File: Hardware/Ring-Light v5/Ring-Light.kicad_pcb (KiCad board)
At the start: 4 copper layers, 115 x 146.1 mm, 319 parts, among them J1 694106301002, J2 1017457000B11LF, J3 U.FL-R-SMT-1_80, J4 2002112100010C4LF, J5 640445-2, J6 Conn_01x01, J7 Conn_01x01, J8 Conn_01x01, J9 Conn_01x01, Q1 SQJ415EP-T1_GE3, U1 NCR321PASX, U10 NCR321PASX, U11 NCR321PASX, U12 NCR321PASX, U13 NCR321PASX, U14 NCR321PASX, U15 NCR321PASX, U16 NCR321PASX, U17 NCR321PASX, U18 NCR321PASX, U19 NCR321PASX, U2 NCR321PASX, U20 NCR321PASX, U21 NCR321PASX, U22 NCR321PASX, U23 NCR321PASX, U24 NCR321PASX, U25 NCR321PASX, U26 NCR321PASX, U27 NCR321PASX, U28 NCR321PASX, U29 NCR321PASX, U3 NCR321PASX, U30 NCR321PASX, U31 NCR321PASX, U32 NCR321PASX, U33 PCA9685BS,118, U34 PCA9685BS,118, U36 TPS62177DQC, U37 CP2102N-A02-GQFN20R, U38 W25X40CLUXIG_TR, U39 CC2640R2FRGZR, U4 NCR321PASX, U5 NCR321PASX, U6 NCR321PASX, U7 NCR321PASX, U8 NCR321PASX, U9 NCR321PASX, Y1 32.768kHz, Y2 24MHz

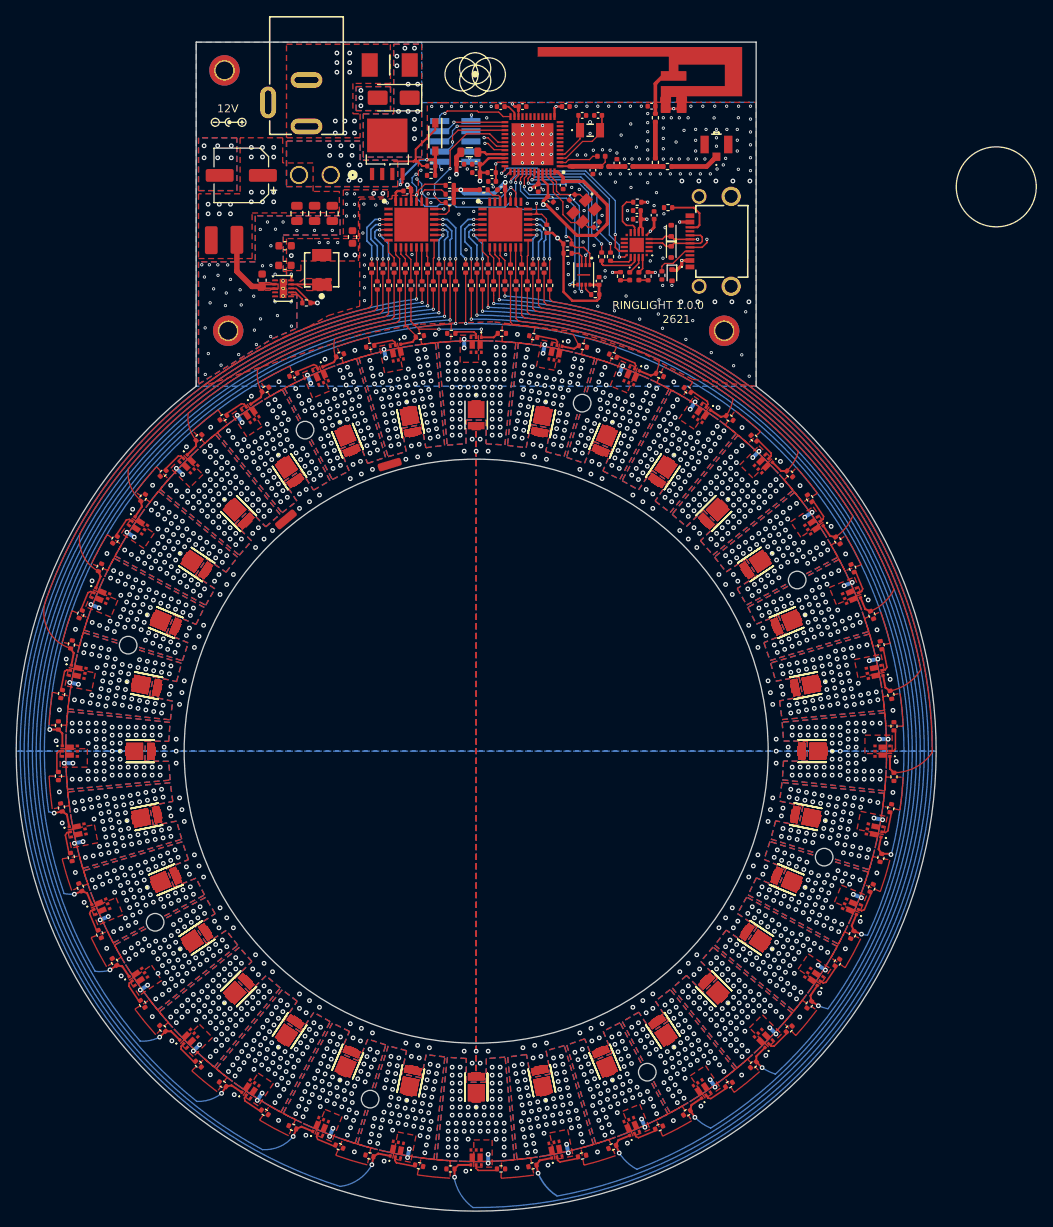
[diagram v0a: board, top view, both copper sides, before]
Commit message: m
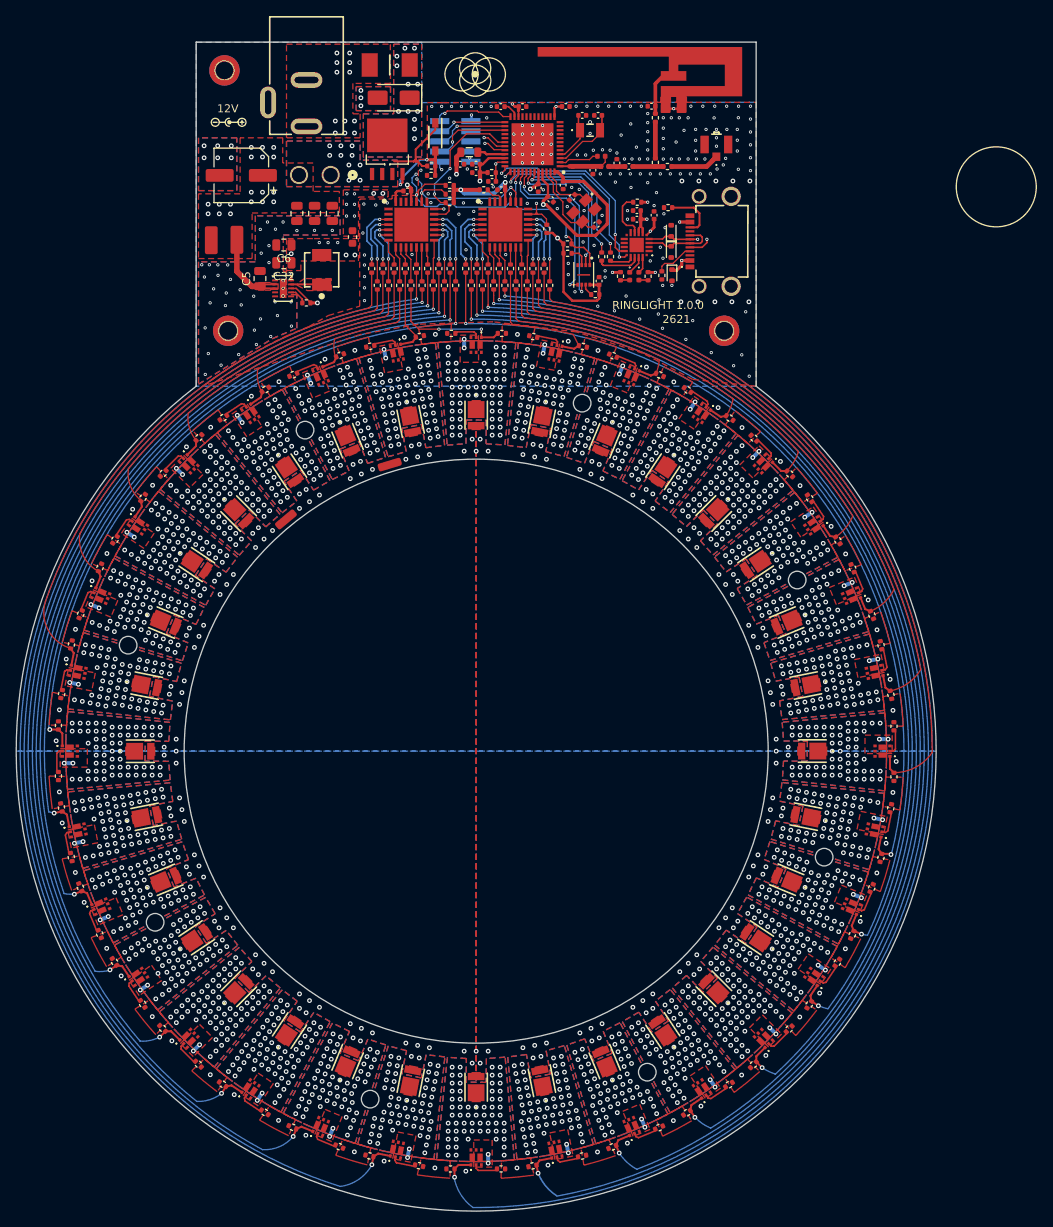
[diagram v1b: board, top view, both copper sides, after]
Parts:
- removed the D10 at (52.9, 126.9) (x2)
- removed the D11 at (55.3, 134.7)
- removed the D12 at (59.2, 142.0)
- removed the D13 at (64.4, 148.4)
- removed the D14 at (70.8, 153.6)
- removed the D15 at (78.1, 157.5)
- removed the D16 at (85.9, 159.9)
- removed the D17 at (94.1, 160.7)
- removed the D18 at (102.3, 159.9)
- removed the D19 at (110.2, 157.5)
- removed the D2 at (85.9, 77.5) (x2)
- removed the D20 at (117.5, 153.6)
- removed the D21 at (123.8, 148.4)
- removed the D22 at (129.0, 142.0) (x2)
- removed the D23 at (132.9, 134.7)
- removed the D24 at (135.3, 126.9) (x2)
- removed the D25 at (136.1, 118.7) (x2)
- removed the D26 at (135.3, 110.5) (x2)
- removed the D27 at (132.9, 102.6) (x2)
- removed the D28 at (129.0, 95.3)
- removed the D29 at (123.8, 89.0)
- removed the D3 at (78.0, 79.9)
- removed the D30 at (117.4, 83.7) (x2)
- removed the D31 at (110.2, 79.9)
- removed the D32 at (102.3, 77.5)
- removed the D4 at (70.8, 83.7)
- removed the D4 at (70.8, 83.8)
- removed D41, D45, D47, D49, D50, D51, D52, D53, D54, D55, D56, D57, D58, D59, D61, D66, D67, D69, D70: LED, Library:GWJTLRS1EMLVL5XX531
- removed the D5 at (64.4, 89.0) (x2)
- removed the D6 at (59.2, 95.3) (x2)
- removed the D7 at (55.3, 102.6)
- removed the D8 at (52.9, 110.5) (x2)
- removed the D9 at (52.1, 118.7)
- C1, C2, C7, C8: value 0.1uF -> 100nF
- C20: value 1.0uF -> 1uF
- C32, C6: footprint Capacitor_SMD:C_0603_1608Metric -> Capacitor_SMD:C_0805_2012Metric
- C5: value 0.1uF -> 2.2uF; footprint Capacitor_SMD:C_0603_1608Metric -> Capacitor_SMD:C_0805_2012Metric
- moved C32 0.35 mm to (70.1, 57.6)
- moved C5 0.34 mm to (67.1, 59.6)
- moved C6 0.18 mm to (70.1, 55.4)
- renumbered D48 to D10, D60 to D22, D62 to D24, D63 to D25, D64 to D26, D65 to D27, D68 to D30, D42 to D4, D43 to D5, D44 to D6, D46 to D8
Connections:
- D10 pad 1: /LEDs_1-16/OUT1 -> /LEDs_1-16/OUT10
- D10 pad 2: /LEDs_1-16/OUT1 -> /LEDs_1-16/OUT10
- D11 pad 1: /LEDs_1-16/OUT1 -> /LEDs_1-16/OUT11
- D11 pad 2: /LEDs_1-16/OUT1 -> /LEDs_1-16/OUT11
- D13 pad 1: /LEDs_1-16/OUT1 -> /LEDs_1-16/OUT13
- D13 pad 2: /LEDs_1-16/OUT1 -> /LEDs_1-16/OUT13
- D16 pad 1: /LEDs_1-16/OUT1 -> /LEDs_1-16/OUT16
- D16 pad 2: /LEDs_1-16/OUT1 -> /LEDs_1-16/OUT16
- D18 pad 1: /LEDs_1-16/OUT1 -> /LEDs_17-32/OUT18
- D18 pad 2: /LEDs_1-16/OUT1 -> /LEDs_17-32/OUT18
- D2 pad 1: /LEDs_1-16/OUT1 -> /LEDs_1-16/OUT2
- D2 pad 2: /LEDs_1-16/OUT1 -> /LEDs_1-16/OUT2
- D21 pad 1: /LEDs_1-16/OUT1 -> /LEDs_17-32/OUT21
- D21 pad 2: /LEDs_1-16/OUT1 -> /LEDs_17-32/OUT21
- D22 pad 1: /LEDs_1-16/OUT1 -> /LEDs_17-32/OUT22
- D22 pad 2: /LEDs_1-16/OUT1 -> /LEDs_17-32/OUT22
- D23 pad 1: /LEDs_1-16/OUT1 -> /LEDs_17-32/OUT23
- D23 pad 2: /LEDs_1-16/OUT1 -> /LEDs_17-32/OUT23
- D24 pad 1: /LEDs_1-16/OUT1 -> /LEDs_17-32/OUT24
- D24 pad 2: /LEDs_1-16/OUT1 -> /LEDs_17-32/OUT24
- D25 pad 1: /LEDs_1-16/OUT1 -> /LEDs_17-32/OUT25
- D25 pad 2: /LEDs_1-16/OUT1 -> /LEDs_17-32/OUT25
- D26 pad 1: /LEDs_1-16/OUT1 -> /LEDs_17-32/OUT26
- D26 pad 2: /LEDs_1-16/OUT1 -> /LEDs_17-32/OUT26
- D27 pad 1: /LEDs_1-16/OUT1 -> /LEDs_17-32/OUT27
- D27 pad 2: /LEDs_1-16/OUT1 -> /LEDs_17-32/OUT27
- D28 pad 1: /LEDs_1-16/OUT1 -> /LEDs_17-32/OUT28
- D28 pad 2: /LEDs_1-16/OUT1 -> /LEDs_17-32/OUT28
- D29 pad 1: /LEDs_1-16/OUT1 -> /LEDs_17-32/OUT29
- D29 pad 2: /LEDs_1-16/OUT1 -> /LEDs_17-32/OUT29
- D30 pad 1: /LEDs_1-16/OUT1 -> /LEDs_17-32/OUT30
- D30 pad 2: /LEDs_1-16/OUT1 -> /LEDs_17-32/OUT30
- D32 pad 1: /LEDs_1-16/OUT1 -> /LEDs_17-32/OUT32
- D32 pad 2: /LEDs_1-16/OUT1 -> /LEDs_17-32/OUT32
- D4 pad 1: /LEDs_1-16/OUT1 -> /LEDs_1-16/OUT4
- D4 pad 2: /LEDs_1-16/OUT1 -> /LEDs_1-16/OUT4
- D5 pad 1: /LEDs_1-16/OUT1 -> /LEDs_1-16/OUT5
- D5 pad 2: /LEDs_1-16/OUT1 -> /LEDs_1-16/OUT5
- D6 pad 1: /LEDs_1-16/OUT1 -> /LEDs_1-16/OUT6
- D6 pad 2: /LEDs_1-16/OUT1 -> /LEDs_1-16/OUT6
- D8 pad 1: /LEDs_1-16/OUT1 -> /LEDs_1-16/OUT8
- D8 pad 2: /LEDs_1-16/OUT1 -> /LEDs_1-16/OUT8
- D9 pad 1: /LEDs_1-16/OUT1 -> /LEDs_1-16/OUT9
- D9 pad 2: /LEDs_1-16/OUT1 -> /LEDs_1-16/OUT9
